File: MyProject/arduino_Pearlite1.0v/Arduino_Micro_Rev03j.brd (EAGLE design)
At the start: 47.8 x 58.3 mm, 46 parts, among them CON1 B3B-ZR, CON2 B3B-ZR, CON3 B3B-ZR, J3 USB-MICRO!!!, J4 3x2M, J5 HEAD17-NOSS, J6 HEAD17-NOSS-1, T1 FDN340P/PMV48XP, T2 PMV48XP, U1 ATMEGA32U4-XUMU, U4 LP2985-33DBVR, Y3 16MHz KX-7

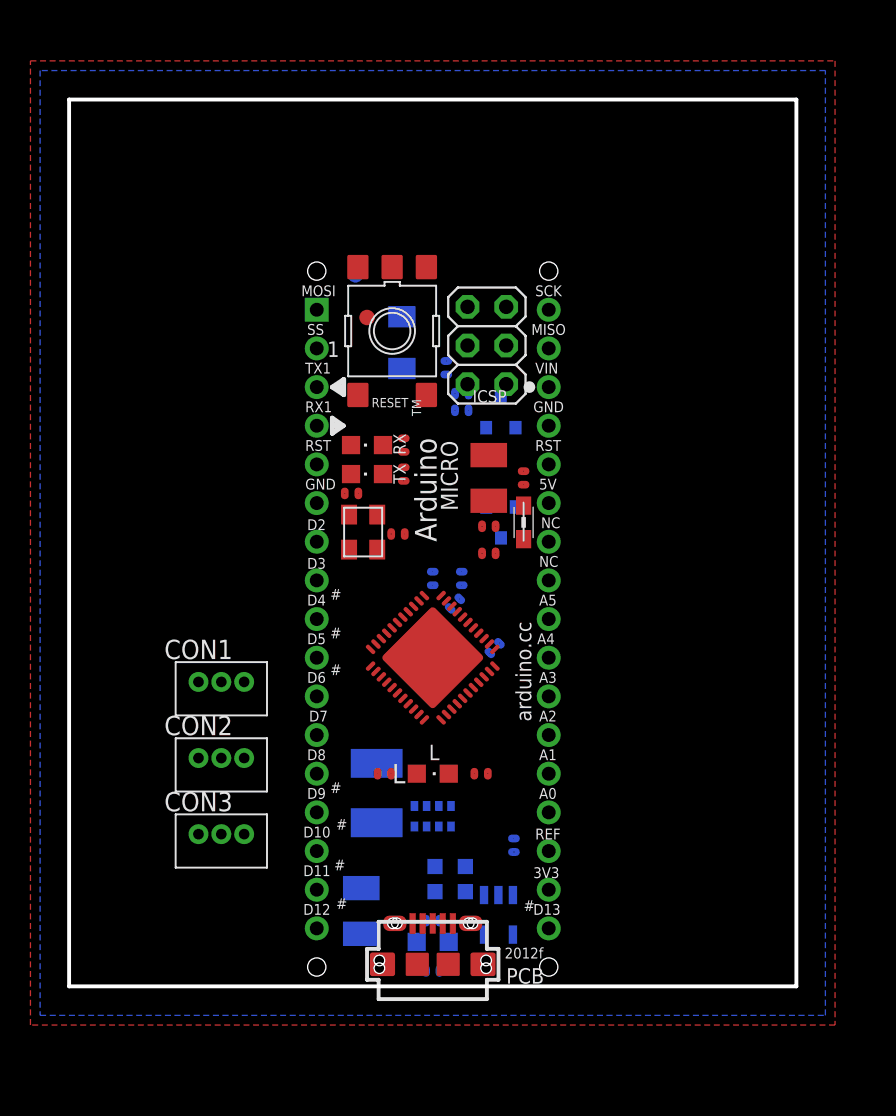
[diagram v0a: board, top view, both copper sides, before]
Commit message: syukujitu syuuryou
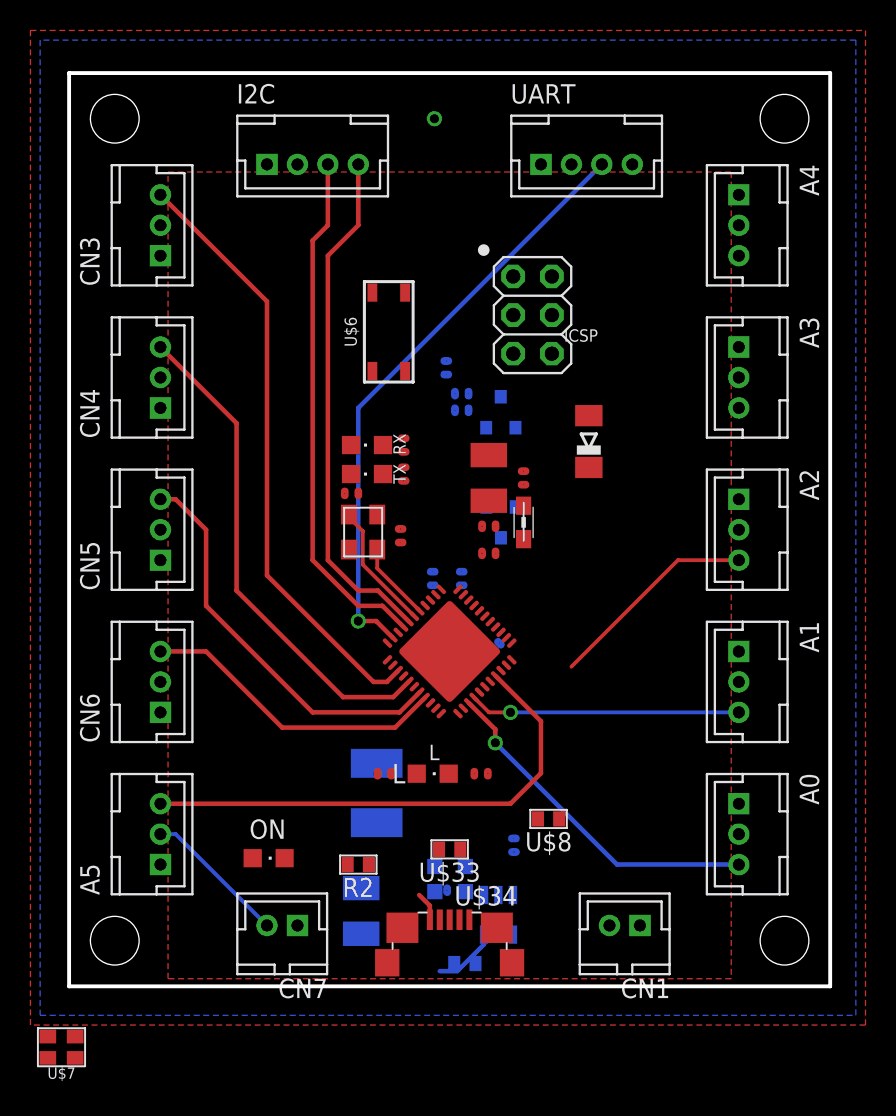
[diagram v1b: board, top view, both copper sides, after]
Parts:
- removed CON1, CON2, CON3: B3B-ZR, jst:B3B-ZR
- removed J3: USB-MICRO!!!, SmartPrj:CON2_USB_MICRO_B_AT
- removed J5: HEAD17-NOSS, SmartPrj:HEAD17-NOSS
- removed J6: HEAD17-NOSS-1, SmartPrj:HEAD17-NOSS-1
- removed RESET: TS42, SmartPrj:TS42
- removed RP3: 22R, resistor-dil:CAY16
- removed U$37: FIDUCIALMOUNT, SmartPrj:FIDUCIA-MOUNT
- removed U$53: FIDUCIAL1X2, SparkFun:FIDUCIAL-1X2
- added A0, A1, A2, A3, A4, A5, CN3, CN4, CN5, CN6: (no value), jst-pa:B3B-PH-K-S
- added CN1, CN7: (no value), jst-pa:B2B-PH-K-S
- added I2C, UART: (no value), jst-pa:B4B-PH-K-S
- added U$33, U$8: (no value), 01_R:1608
- added U$34: MICRO-USB-SHIELD-ZX62R-B-5P, con-hirose1:ZX62R-B-5P
- added U$6: SKRPACE010, 09_1_switch:SKRP
- added U$7: X22, 09_2_CRYSTAL:SMD_X22
- C4: value 1uF -> (none); device SmartPrj:C0402 -> 02_C:1608
- R2: value 10K -> (none); device SmartPrj:R0402 -> 01_R:1608
- moved R2 18.3 mm to (19.0, 8.00), flipped to the top, turned to 0 degrees
- moved D2 13.9 mm to (34.1, 35.8), flipped to the top
- moved ON 12.1 mm to (13.1, 8.42), flipped to the top
- moved J4 3.61 mm to (30.4, 44.1)
- moved C4 2.16 mm to (26.0, 1.50), turned to 180 degrees
- moved R5 2.06 mm to (24.4, 6.32)
- moved U1 1.18 mm to (25.0, 22.0)
- moved C12 0.21 mm to (21.8, 29.6), turned to 270 degrees
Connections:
- removed net 5-GND: RESET.5
- net +5V: now also A0.2, A1.2, A2.2, A3.2, A4.2, A5.2, CN3.2, CN4.2, CN5.2, CN6.2, CN7.2, I2C.2, UART.2; no longer J6.6
- net 3V3: now also C4.P$1; no longer C4.1, J6.16
- net A0: now also A0.3; no longer J6.14
- net A1: now also A1.3; no longer J6.13
- net A2: now also A2.3; no longer J6.12
- net A3: now also A3.3; no longer J6.11
- net A4: now also A4.3; no longer J6.10
- net A5: now also A5.3; no longer J6.9
- net AREF: no longer J6.15
- net D+: now also U$33.1, U$34.3; no longer J3.P3, RP3.8
- net D-: now also U$34.2, U$8.1; no longer J3.P2, RP3.7
- net D0/RX: now also UART.4; no longer J5.4
- net D1/TX: now also UART.3; no longer J5.3
- net D2/SDA: now also I2C.3; no longer J5.7
- net D3/SCL: now also I2C.4; no longer J5.8
- net D4*: now also CN3.3; no longer J5.9
- net D5*: no longer J5.10
- net D6*: now also CN4.3; no longer J5.11
- net D7: no longer J5.12
- net GND: now also A0.1, A1.1, A2.1, A3.1, A4.1, A5.1, C4.P$2, CN3.1, CN4.1, CN5.1, CN6.1, CN7.1, I2C.1, U$34.5, U$34.M1, U$34.M2, U$34.M3, U$34.M4, U$6.3, U$6.4, UART.1; no longer C4.2, J3.P5, J3.S1, J3.S2, J3.S3, J3.S4, J3.S5, J3.S6, J5.6, J6.4, RESET.3, RESET.4, RP3.3, RP3.4, RP3.5, RP3.6
- net IO10*: now also CN6.3; no longer J5.15
- net IO11*: no longer J5.16
- net IO12*: no longer J5.17
- net IO13*: no longer J6.17
- net IO8: no longer J5.13
- net IO9*: now also CN5.3; no longer J5.14
- net MISO: no longer J6.2
- net MOSI: no longer J5.1
- net RD+: now also U$33.2; no longer RP3.1
- net RD-: now also U$8.2; no longer RP3.2
- net RESET: now also U$6.1, U$6.2; no longer J5.5, J6.5, RESET.2
- net RXLED/SS: no longer J5.2
- net SCK: no longer J6.1
- net VIN: no longer J6.3
- net VUSBD: now also U$34.1; no longer J3.P1
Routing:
- net D4*: track 0.00 -> 39.7 mm
- net D1/TX: track 0.00 -> 39.4 mm, vias 0 -> 1
- net D2/SDA: track 0.00 -> 34.2 mm
- net D3/SCL: track 0.00 -> 33.8 mm
- net A5: track 0.00 -> 33.5 mm
- net D6*: track 0.00 -> 32.7 mm
- net IO9*: track 0.00 -> 26.3 mm
- net A0: track 0.00 -> 22.7 mm, vias 0 -> 1
- net IO10*: track 0.00 -> 20.3 mm
- net A1: track 0.00 -> 17.8 mm, vias 0 -> 1
- net A2: track 0.00 -> 13.9 mm
- net +5V: track 0.00 -> 9.49 mm
- net XTAL1: track 0.00 -> 8.46 mm
- net XTAL2: track 0.00 -> 5.18 mm
- net 3V3: track 0.00 -> 4.28 mm
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- added copper zone on layer 1, net +5V
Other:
- board size 47.8 x 58.3 mm -> 50 x 60 mm
- board text removed: "#"
- board text removed: "1"
- board text removed: "2012f"
- board text removed: "3V3"
- board text removed: "A0"
- board text removed: "A1"
- board text removed: "A2"
- board text removed: "A3"
- board text removed: "A4"
- board text removed: "A5"
- board text removed: "Arduino"
- board text removed: "D10"
- board text removed: "D11"
- board text removed: "D12"
- board text removed: "D13"
- board text removed: "D2"
- board text removed: "D3"
- board text removed: "D4"
- board text removed: "D5"
- board text removed: "D6"
- board text removed: "D7"
- board text removed: "D8"
- board text removed: "D9"
- board text removed: "MICRO"
- board text removed: "MISO"
- board text removed: "MOSI"
- board text removed: "NC"
- board text removed: "REF"
- board text removed: "RST"
- board text removed: "RX1"
- board text removed: "SCK"
- board text removed: "SS"
- board text removed: "TM"
- board text removed: "TX1"
- board text removed: "VIN"
- board text removed: "arduino.cc"
